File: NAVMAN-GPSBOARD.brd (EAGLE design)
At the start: 90.9 x 72.1 mm, 18 parts, among them X2 SMA-142-0701-801/806

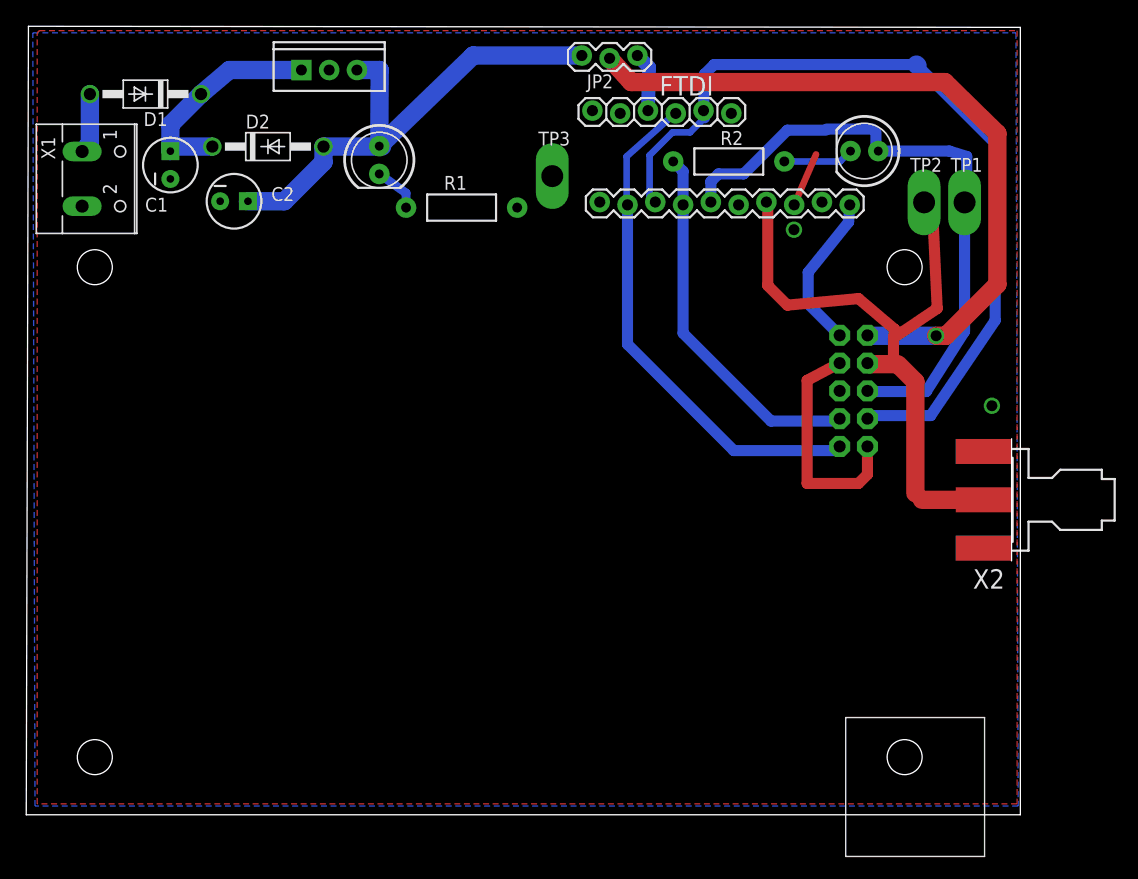
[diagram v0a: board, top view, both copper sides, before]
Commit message: Updated... generated gerbers
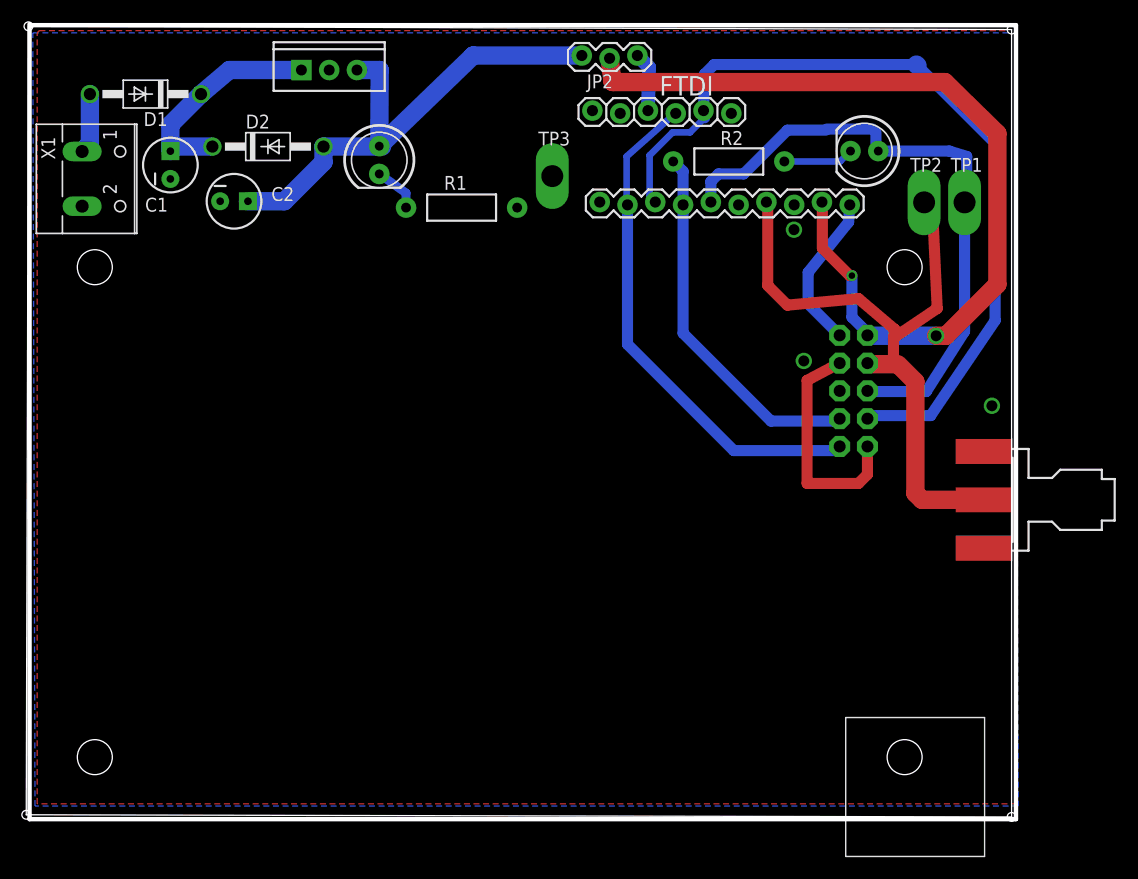
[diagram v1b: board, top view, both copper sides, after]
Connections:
- removed net PWR: JP1.2
- net VSUP: now also JP1.2
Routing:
- net VSUP: track 66.0 -> 81.0 mm, vias 1 -> 2
- net GND: track 26.2 -> 21.2 mm, vias 2 -> 3
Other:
- board size 90.9 x 72.1 mm -> 90.5 x 72.7 mm
- board text added: "Design by Jason Ball (jason@ball.net)"
- board text added: "GPS Disciplined Oscillator"
- board text added: "Navman Jupiter Tu60"
- board text added: "https://github.com/agronaught/GPS-Disciplined-Oscillator-GPSOXCO-.git"
